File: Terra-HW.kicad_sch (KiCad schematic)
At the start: 4 parts

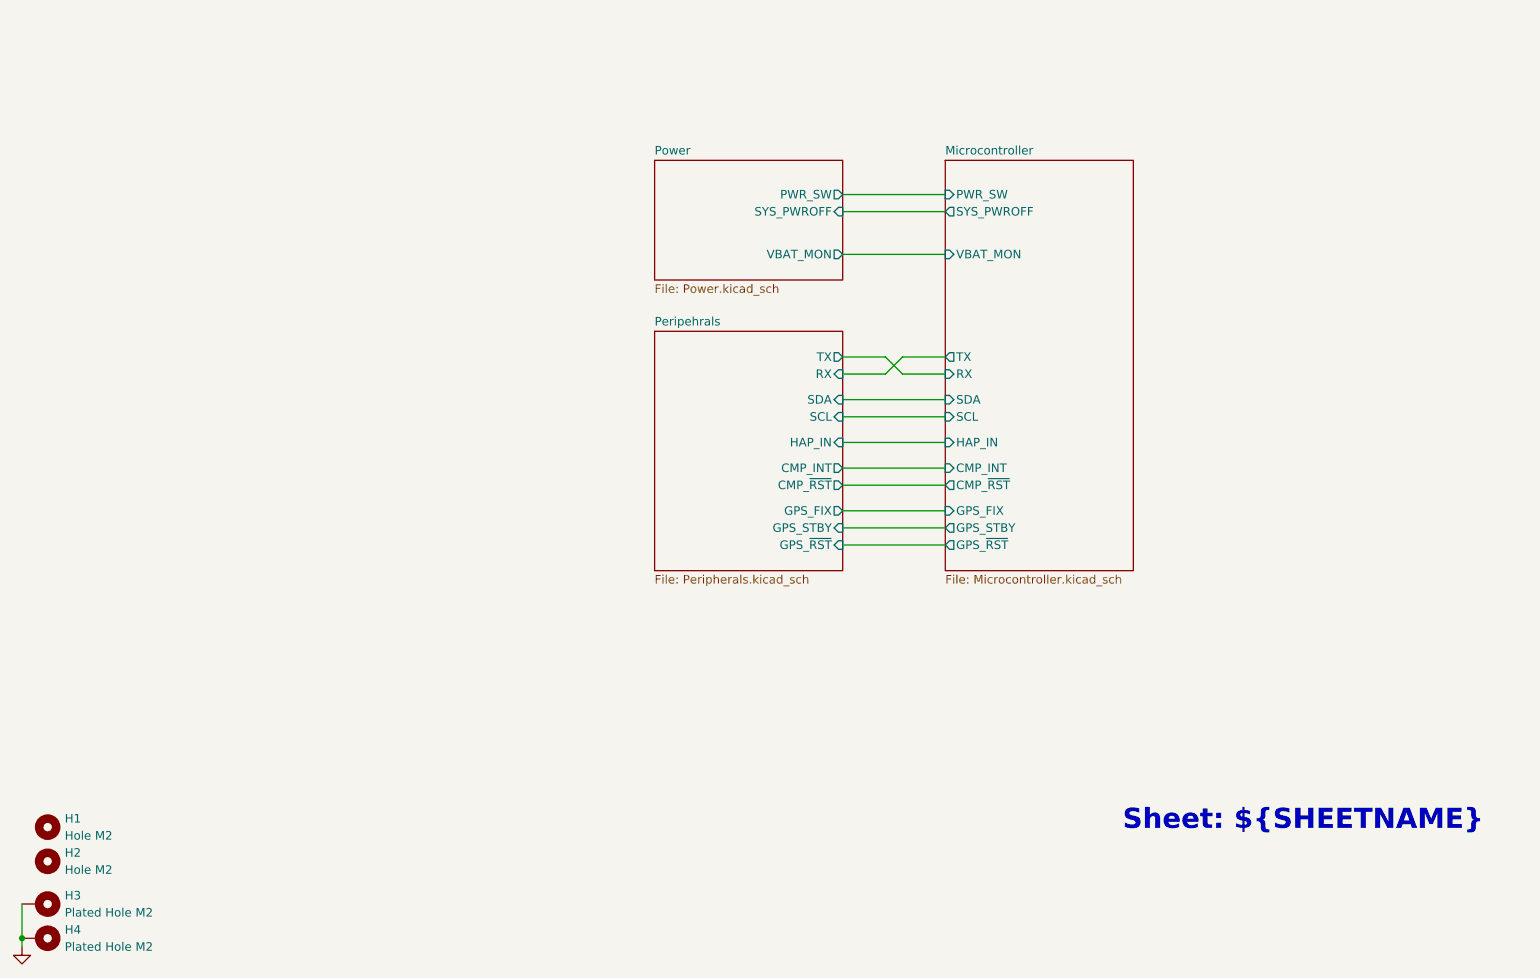
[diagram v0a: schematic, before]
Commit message: Lots of board layout
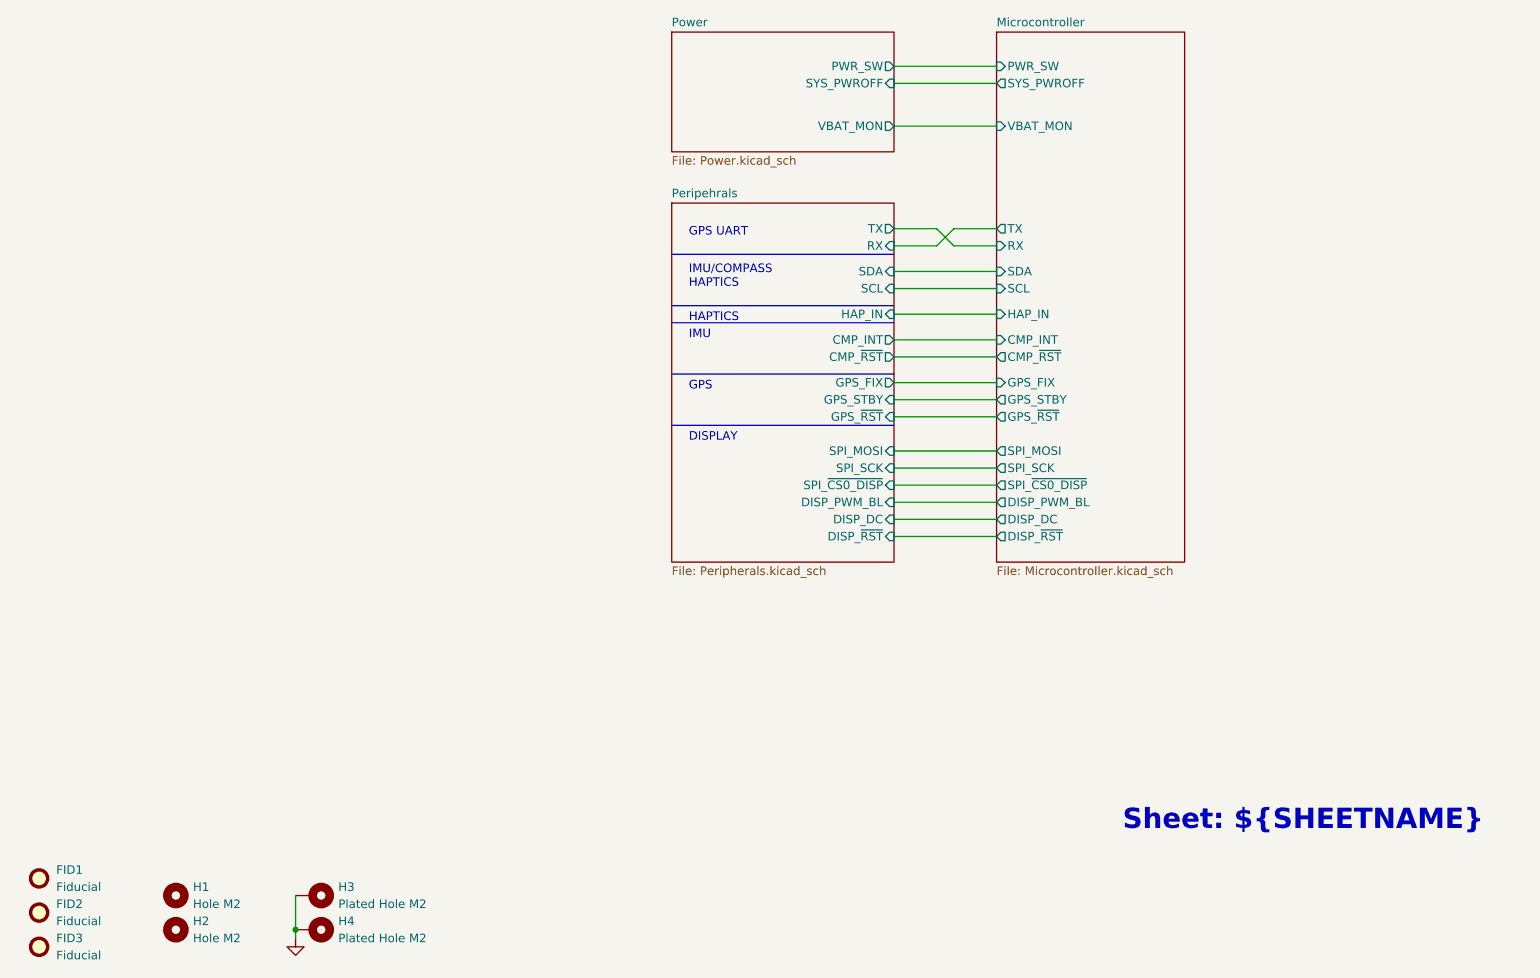
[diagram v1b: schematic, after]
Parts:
- added FID1, FID2, FID3: Fiducial, Fiducial:Fiducial_1mm_Mask2mm, symbol Mechanical:Fiducial
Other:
- sheet Microcontroller ports: added DISP_DC, DISP_PWM_BL, DISP_~{RST}, SPI_MOSI, SPI_SCK, SPI_~{CS0_DISP}; removed none
- sheet Peripehrals ports: added DISP_DC, DISP_PWM_BL, DISP_~{RST}, SPI_MOSI, SPI_SCK, SPI_~{CS0_DISP}; removed none
- note added: "DISPLAY"
- note added: "GPS"
- note added: "GPS UART"
- note added: "HAPTICS"
- note added: "IMU"
- note added: "IMU/COMPASS HAPTICS"
- moved on the sheet: H1, H2, H3, H4
